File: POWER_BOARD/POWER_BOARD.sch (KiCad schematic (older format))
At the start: 37 parts, among them IC1 ILQ30, J1 EXTIN, J2 ARM, J3 Pyro1, J4 Pyro2, J5 Servo2, J6 Servo1, J7 Batt, Q1 IRL40B212, Q2 IRL40B212, U1 SF-1206HH10M-2, U2 SF-1206HH10M-2, U3 AS358AP

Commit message: Update POWER_BOARD.sch
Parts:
- U1, U2: symbol KRTEK_V2:SF-1206HH10M-2 -> POWER_BOARD-rescue:SF-1206HH10M-2-KRTEK_V2
- U3: symbol KRTEK_V2:AS358AP -> POWER_BOARD-rescue:AS358AP-KRTEK_V2
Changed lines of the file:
@@
 	1850 2750 1850 2800
 $Comp
-L KRTEK_V2:AS358AP U3
+L POWER_BOARD-rescue:AS358AP-KRTEK_V2 U3
 U 1 1 617A35D3
 P 9400 1850
@@
 	4850 4600 4550 4600
 $Comp
-L KRTEK_V2:SF-1206HH10M-2 U1
+L POWER_BOARD-rescue:SF-1206HH10M-2-KRTEK_V2 U1
 U 1 1 6198B2D9
 P 4350 4100
@@
 $EndComp
 $Comp
-L KRTEK_V2:SF-1206HH10M-2 U2
+L POWER_BOARD-rescue:SF-1206HH10M-2-KRTEK_V2 U2
 U 1 1 6198C1F2
 P 4350 4550

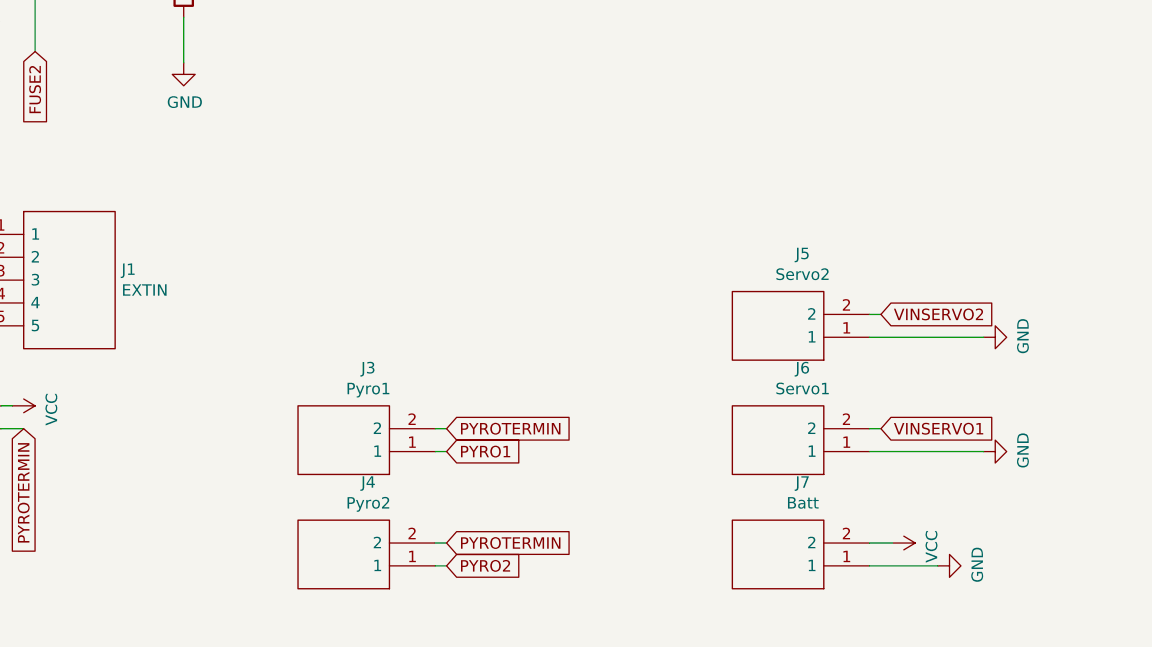
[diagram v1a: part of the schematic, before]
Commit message: duh
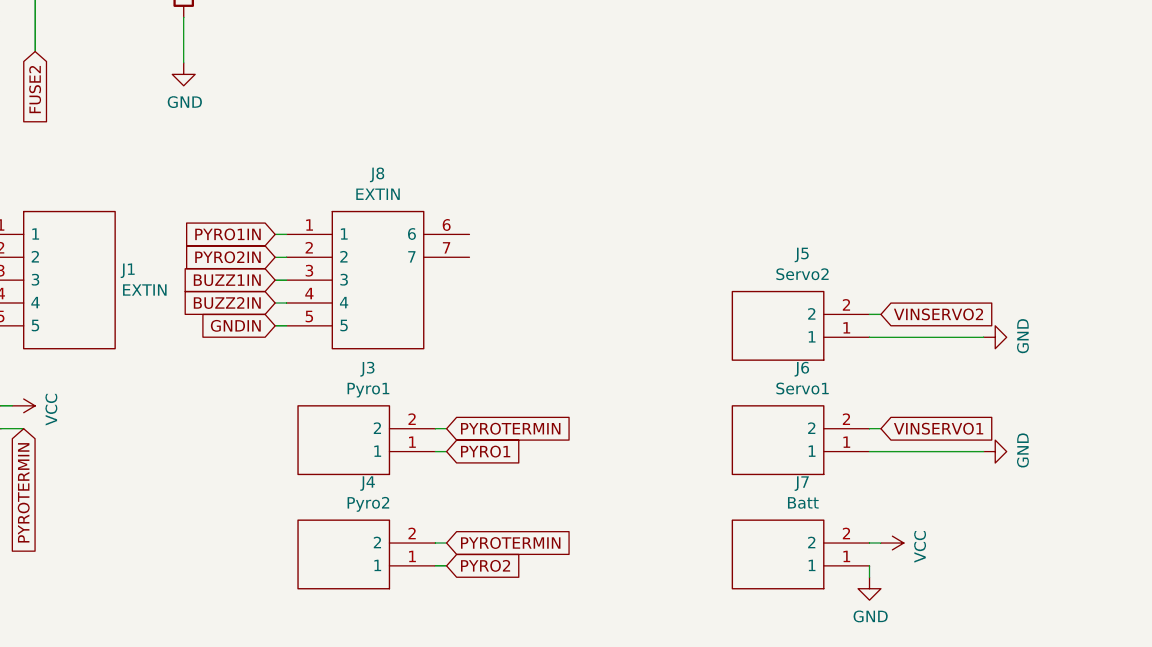
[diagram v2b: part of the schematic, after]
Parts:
- added J8: EXTIN, EXTENSION:5055670571, symbol EXTENSION:505567-0571
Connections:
- net BUZZ1IN: now also J8.3
- net BUZZ2IN: now also J8.4
- net GNDIN: now also J8.5
- net PYRO1IN: now also J8.1
- net PYRO2IN: now also J8.2
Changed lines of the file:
@@
 Text GLabel 3650 7500 2    50   Input ~ 0
 PYRO2
-Wire Wire Line
-	5600 7400 5500 7400
 $Comp
 L power:VCC #PWR016
 U 1 1 61877079
-P 5600 7400
-F 0 "#PWR016" H 5600 7250 50  0001 C CNN
-F 1 "VCC" H 5615 7573 50  0000 C CNN
-F 2 "" H 5600 7400 50  0001 C CNN
-F 3 "" H 5600 7400 50  0001 C CNN
-	1    5600 7400
+P 5550 7400
+F 0 "#PWR016" H 5550 7250 50  0001 C CNN
+F 1 "VCC" H 5565 7573 50  0000 C CNN
+F 2 "" H 5550 7400 50  0001 C CNN
+F 3 "" H 5550 7400 50  0001 C CNN
+	1    5550 7400
 	0    1    1    0
 $EndComp
@@
 L power:GND #PWR017
 U 1 1 61877E3F
-P 5800 7500
-F 0 "#PWR017" H 5800 7250 50  0001 C CNN
-F 1 "GND" H 5805 7327 50  0000 C CNN
-F 2 "" H 5800 7500 50  0001 C CNN
-F 3 "" H 5800 7500 50  0001 C CNN
-	1    5800 7500
-	0    -1   -1   0
-$EndComp
-Wire Wire Line
-	5500 7500 5800 7500
+P 5500 7550
+F 0 "#PWR017" H 5500 7300 50  0001 C CNN
+F 1 "GND" H 5505 7377 50  0000 C CNN
+F 2 "" H 5500 7550 50  0001 C CNN
+F 3 "" H 5500 7550 50  0001 C CNN
+	1    5500 7550
+	1    0    0    -1
+$EndComp
 $Comp
 L SamacSys_Parts:RPM5.0-6.0 PS1
@@
 	1    0    0    -1
 $EndComp
+Wire Wire Line
+	5500 7500 5500 7550
+Wire Wire Line
+	5550 7400 5500 7400
+$Comp
+L EXTENSION:505567-0571 J8
+U 1 1 61909209
+P 2950 6050
+F 0 "J8" H 3350 6315 50  0000 C CNN
+F 1 "EXTIN" H 3350 6224 50  0000 C CNN
+F 2 "EXTENSION:5055670571" H 3600 6150 50  0001 L CNN
+F 3 "https://www.molex.com/pdm_docs/sd/5055670571_sd.pdf" H 3600 6050 50  0001 L CNN
+F 4 "Molex Micro-Lock PLUS 505567, 1.25mm Pitch, 5 Way, 1 Row, Right Angle PCB Header, Surface Mount" H 3600 5950 50  0001 L CNN "Description"
+F 5 "3" H 3600 5850 50  0001 L CNN "Height"
+F 6 "538-505567-0571" H 3600 5750 50  0001 L CNN "Mouser Part Number"
+F 7 "https://www.mouser.co.uk/ProductDetail/Molex/505567-0571?qs=gt1LBUVyoHnJxHrzoS78pw%3D%3D" H 3600 5650 50  0001 L CNN "Mouser Price/Stock"
+F 8 "Molex" H 3600 5550 50  0001 L CNN "Manufacturer_Name"
+F 9 "505567-0571" H 3600 5450 50  0001 L CNN "Manufacturer_Part_Number"
+	1    2950 6050
+	1    0    0    -1
+$EndComp
+Text GLabel 2900 6050 0    50   Input ~ 0
+PYRO1IN
+Text GLabel 2900 6150 0    50   Input ~ 0
+PYRO2IN
+Text GLabel 2900 6250 0    50   Input ~ 0
+BUZZ1IN
+Text GLabel 2900 6350 0    50   Input ~ 0
+BUZZ2IN
+Text GLabel 2900 6450 0    50   Input ~ 0
+GNDIN
+Wire Wire Line
+	2900 6450 2950 6450
+Wire Wire Line
+	2900 6350 2950 6350
+Wire Wire Line
+	2900 6250 2950 6250
+Wire Wire Line
+	2900 6150 2950 6150
+Wire Wire Line
+	2900 6050 2950 6050
 $EndSCHEMATC

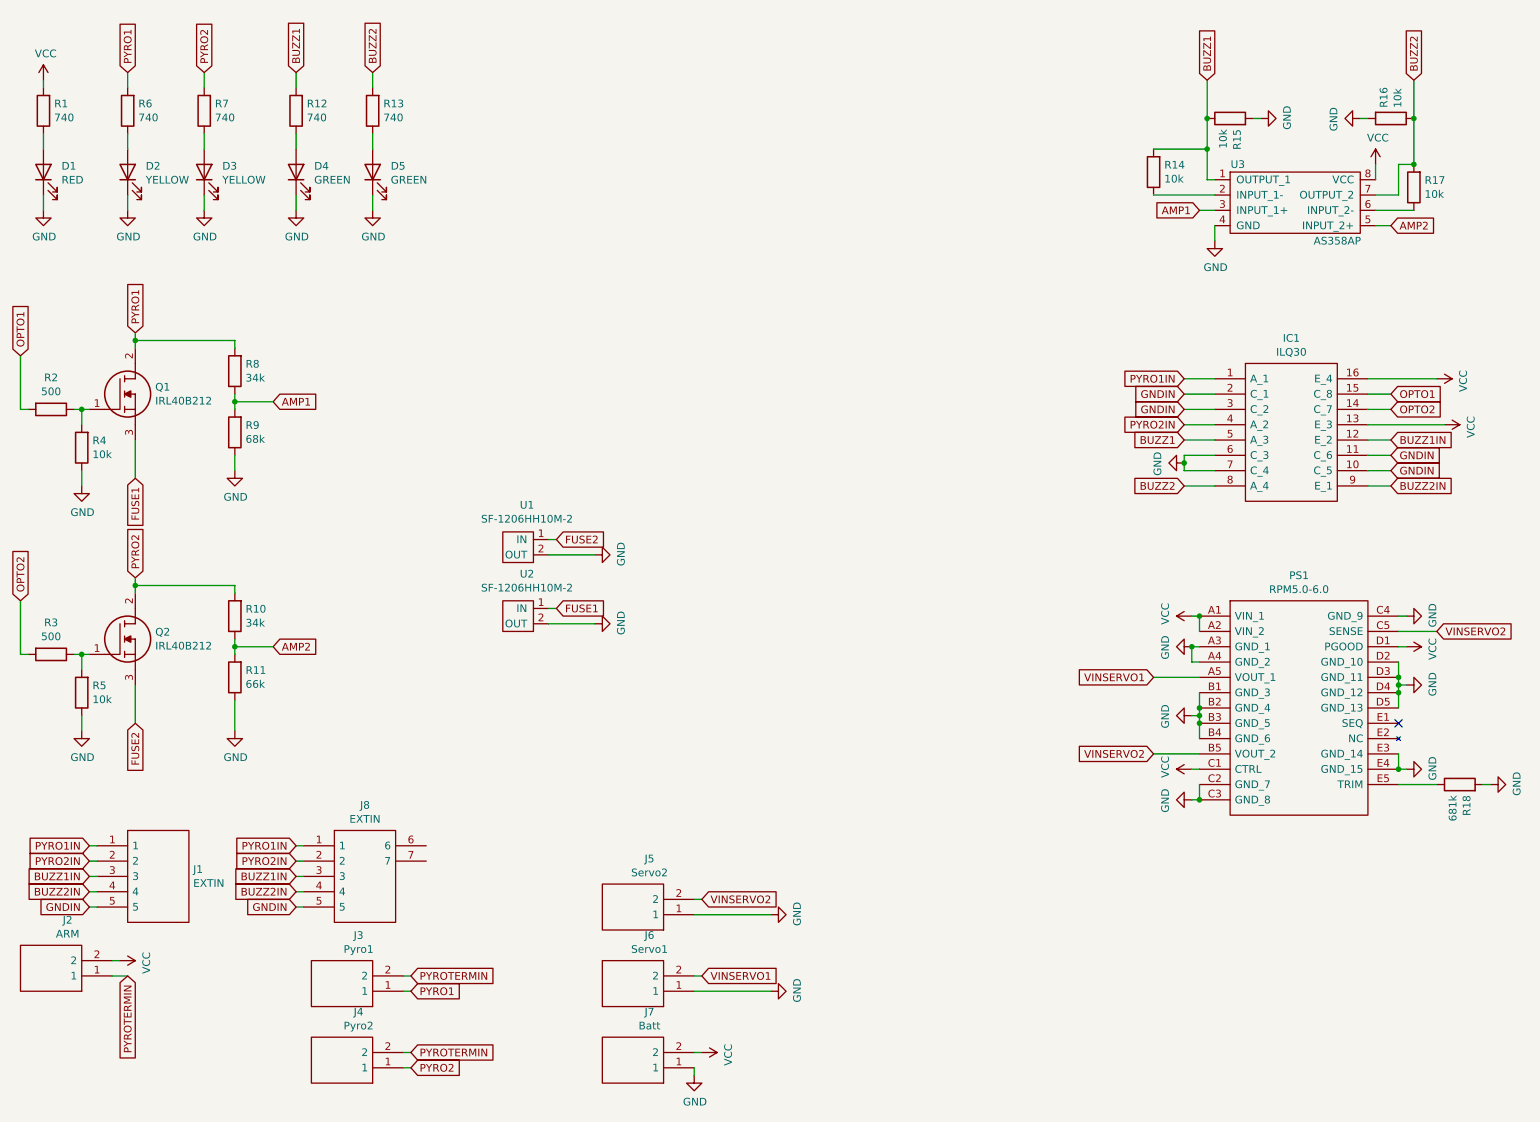
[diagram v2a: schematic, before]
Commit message: Worked again
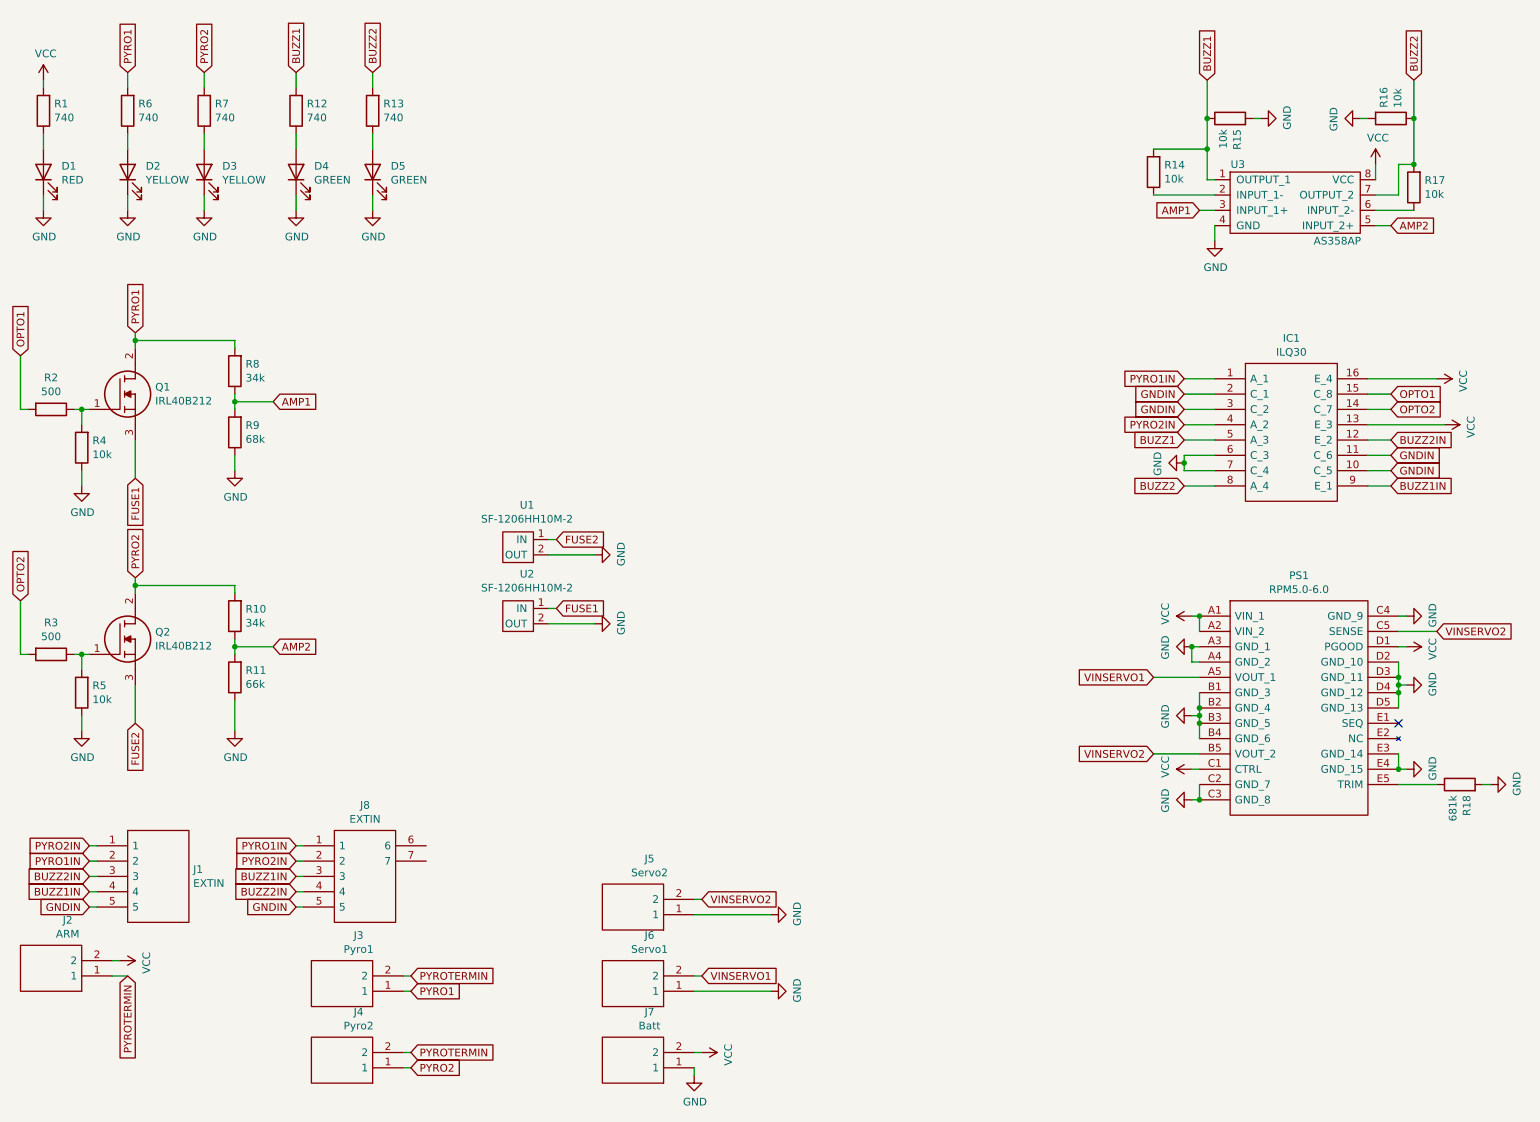
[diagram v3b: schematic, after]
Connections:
- net BUZZ1IN: now also IC1.9 (E_1), J1.4; no longer IC1.12 (E_2), J1.3
- net BUZZ2IN: now also IC1.12 (E_2), J1.3; no longer IC1.9 (E_1), J1.4
- net PYRO1IN: now also J1.2; no longer J1.1
- net PYRO2IN: now also J1.1; no longer J1.2
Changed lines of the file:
@@
 Text GLabel 8700 3300 0    50   Input ~ 0
 PYRO2IN
-Text GLabel 10050 3400 2    50   Input ~ 0
+Text GLabel 10050 3700 2    50   Input ~ 0
 BUZZ1IN
 Text GLabel 10050 3500 2    50   Input ~ 0
@@
 Text GLabel 10050 3600 2    50   Input ~ 0
 GNDIN
-Text GLabel 10050 3700 2    50   Input ~ 0
+Text GLabel 10050 3400 2    50   Input ~ 0
 BUZZ2IN
 Wire Wire Line
@@
 Wire Wire Line
 	9900 1300 9850 1300
+Text GLabel 1550 6150 0    50   Input ~ 0
+PYRO1IN
 Text GLabel 1550 6050 0    50   Input ~ 0
-PYRO1IN
-Text GLabel 1550 6150 0    50   Input ~ 0
 PYRO2IN
+Text GLabel 1550 6350 0    50   Input ~ 0
+BUZZ1IN
 Text GLabel 1550 6250 0    50   Input ~ 0
-BUZZ1IN
-Text GLabel 1550 6350 0    50   Input ~ 0
 BUZZ2IN
 Text GLabel 1550 6450 0    50   Input ~ 0
